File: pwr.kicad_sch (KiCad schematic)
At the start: 25 parts, among them U2 AMS1117-3.3, U4 TPS54336ADDA

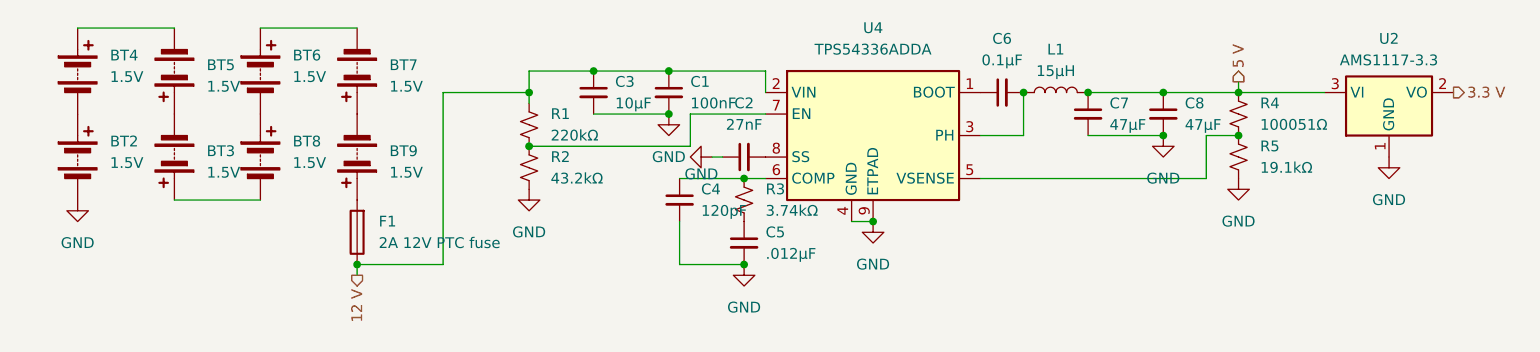
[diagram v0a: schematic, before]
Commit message: Modifications to power system to support what is required
modified
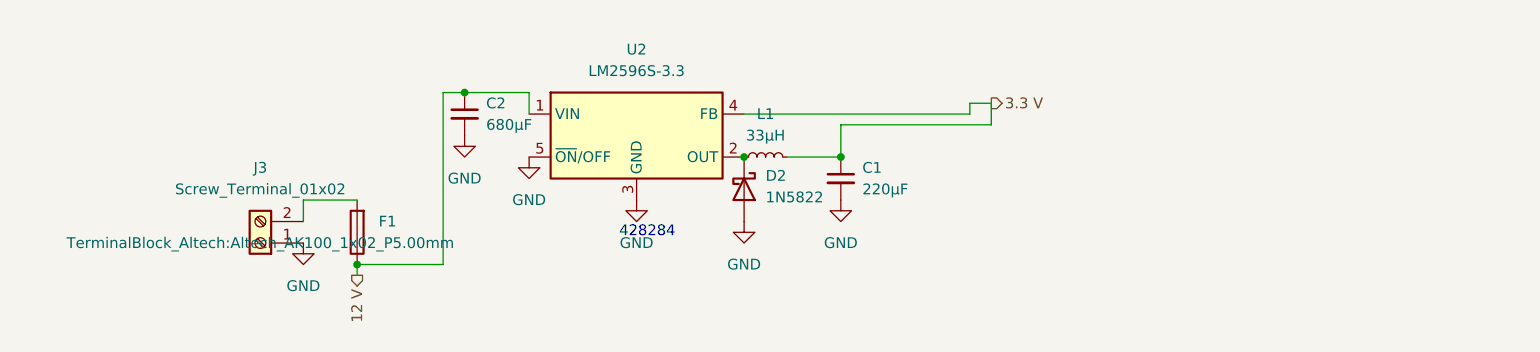
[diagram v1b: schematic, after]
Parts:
- removed BT2, BT3, BT4, BT5, BT6, BT7, BT8, BT9: 1.5V, symbol Device:Battery
- removed C3: 10µF, Capacitor_SMD:C_0603_1608Metric, symbol Device:C_Small
- removed C4: 120pF, Capacitor_SMD:C_0603_1608Metric, symbol Device:C_Small
- removed C5: .012µF, Capacitor_SMD:C_0603_1608Metric, symbol Device:C_Small
- removed C6: 0.1µF, Capacitor_SMD:C_0603_1608Metric, symbol Device:C_Small
- removed C7, C8: 47µF, Capacitor_SMD:C_0603_1608Metric, symbol Device:C_Small
- removed L1: 15µH, Capacitor_SMD:C_0603_1608Metric, symbol Device:L
- removed R1: 220kΩ, Resistor_SMD:R_0603_1608Metric, symbol Device:R_Small_US
- removed R2: 43.2kΩ, Resistor_SMD:R_0603_1608Metric, symbol Device:R_Small_US
- removed R3: 3.74kΩ, Resistor_SMD:R_0603_1608Metric, symbol Device:R_Small_US
- removed R4: 100051Ω, Resistor_SMD:R_0603_1608Metric, symbol Device:R_Small_US
- removed R5: 19.1kΩ, Resistor_SMD:R_0603_1608Metric, symbol Device:R_Small_US
- removed U2: AMS1117-3.3, Package_TO_SOT_SMD:SOT-223-3_TabPin2, symbol Regulator_Linear:AMS1117-3.3
- removed U4: TPS54336ADDA, Package_SO:TI_SO-PowerPAD-8_ThermalVias, symbol Regulator_Switching:TPS54336ADDA
- added D2: 1N5822, Diode_THT:D_DO-201AD_P15.24mm_Horizontal, symbol Diode:1N5822
- added J3: Screw_Terminal_01x02, TerminalBlock_Altech:Altech_AK100_1x02_P5.00mm, symbol Connector:Screw_Terminal_01x02
- added L1: 33µH, symbol Device:L_Small
- added U2: LM2596S-3.3, Package_TO_SOT_SMD:TO-263-5_TabPin3, symbol Regulator_Switching:LM2596S-3.3
- C1: value 100nF -> 220µF; footprint Capacitor_SMD:C_0603_1608Metric -> (none)
- C2: value 27nF -> 680µF; footprint Capacitor_SMD:C_0603_1608Metric -> (none)
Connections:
- net 12 V: now also C2.1, U2.1 (VIN); no longer C1.1
- net 3.3 V: now also C1.1, L1.2, U2.4 (FB)
- net GND: now also C2.2, D2.2 (A), J3.1 (Pin_1), U2.3 (GND), U2.5 (~{ON}/OFF); no longer C2.1
- net at F1.2: now also J3.2 (Pin_2)
- new net: D2.1 (K), L1.1, U2.2 (OUT)
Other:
- note added: "428284"
